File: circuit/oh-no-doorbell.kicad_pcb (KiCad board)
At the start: 2 copper layers, 3.6 x 3.4 mm, 2 parts, among them J2 Conn_VDG, U1 ATtiny4-TS

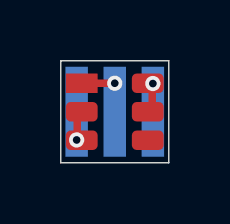
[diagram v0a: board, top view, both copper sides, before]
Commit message: Fix PCB
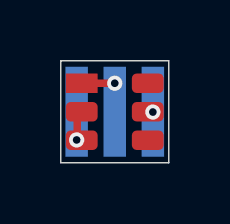
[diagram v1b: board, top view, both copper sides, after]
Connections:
- U1 pad 6: /BJT_C -> Net-(U1-Pad6)
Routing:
- net /BJT_C: track 1.07 -> 0.00 mm
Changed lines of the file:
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@@
     (thickness 0.2)
     (drawings 4)
-    (tracks 10)
+    (tracks 7)
     (zones 0)
     (modules 2)
-    (nets 5)
+    (nets 6)
   )
   (page A4)
@@
     (pad_to_mask_clearance 0)
     (aux_axis_origin 0 0)
-    (visible_elements 7FFFFFFF)
+    (visible_elements 7FFFFF7F)
     (pcbplotparams
       (layerselection 0x010fc_ffffffff)
@@
   (net 3 /BJT_E)
   (net 4 "Net-(U1-Pad4)")
+  (net 5 "Net-(U1-Pad6)")
   (net_class Default "This is the default net class."
     (clearance 0.2)
@@
     (add_net /BJT_E)
     (add_net "Net-(U1-Pad4)")
+    (add_net "Net-(U1-Pad6)")
   )
   (module Package_TO_SOT_SMD:SOT-23-6 (layer F.Cu)
@@
       (effects (font (size 1 1) (thickness 0.15)))
     )
-    (fp_line (start 0.9 -1.55) (end 0.9 1.55) (layer F.Fab) (width 0.1))
-    (fp_line (start 0.9 1.55) (end -0.9 1.55) (layer F.Fab) (width 0.1))
-    (fp_line (start -0.9 -0.9) (end -0.9 1.55) (layer F.Fab) (width 0.1))
-    (fp_line (start 0.9 -1.55) (end -0.25 -1.55) (layer F.Fab) (width 0.1))
-    (fp_line (start -0.9 -0.9) (end -0.25 -1.55) (layer F.Fab) (width 0.1))
-    (fp_line (start -1.9 -1.8) (end -1.9 1.8) (layer F.CrtYd) (width 0.05))
-    (fp_line (start -1.9 1.8) (end 1.9 1.8) (layer F.CrtYd) (width 0.05))
-    (fp_line (start 1.9 1.8) (end 1.9 -1.8) (layer F.CrtYd) (width 0.05))
-    (fp_line (start 1.9 -1.8) (end -1.9 -1.8) (layer F.CrtYd) (width 0.05))
     (fp_text user %R (at 0 0 90) (layer F.Fab) hide
       (effects (font (size 0.5 0.5) (thickness 0.075)))
     )
+    (fp_line (start 1.9 -1.8) (end -1.9 -1.8) (layer F.CrtYd) (width 0.05))
+    (fp_line (start 1.9 1.8) (end 1.9 -1.8) (layer F.CrtYd) (width 0.05))
+    (fp_line (start -1.9 1.8) (end 1.9 1.8) (layer F.CrtYd) (width 0.05))
+    (fp_line (start -1.9 -1.8) (end -1.9 1.8) (layer F.CrtYd) (width 0.05))
+    (fp_line (start -0.9 -0.9) (end -0.25 -1.55) (layer F.Fab) (width 0.1))
+    (fp_line (start 0.9 -1.55) (end -0.25 -1.55) (layer F.Fab) (width 0.1))
+    (fp_line (start -0.9 -0.9) (end -0.9 1.55) (layer F.Fab) (width 0.1))
+    (fp_line (start 0.9 1.55) (end -0.9 1.55) (layer F.Fab) (width 0.1))
+    (fp_line (start 0.9 -1.55) (end 0.9 1.55) (layer F.Fab) (width 0.1))
+    (pad 1 smd rect (at -1.1 -0.95) (size 1.06 0.65) (layers F.Cu F.Paste F.Mask)
+      (net 1 /BJT_B))
+    (pad 2 smd roundrect (at -1.1 0) (size 1.06 0.65) (layers F.Cu F.Paste F.Mask) (roundrect_rratio 0.25)
+      (net 3 /BJT_E))
+    (pad 3 smd roundrect (at -1.1 0.95) (size 1.06 0.65) (layers F.Cu F.Paste F.Mask) (roundrect_rratio 0.25)
+      (net 3 /BJT_E))
+    (pad 4 smd roundrect (at 1.1 0.95) (size 1.06 0.65) (layers F.Cu F.Paste F.Mask) (roundrect_rratio 0.25)
+      (net 4 "Net-(U1-Pad4)"))
+    (pad 6 smd roundrect (at 1.1 -0.95) (size 1.06 0.65) (layers F.Cu F.Paste F.Mask) (roundrect_rratio 0.25)
+      (net 5 "Net-(U1-Pad6)"))
     (pad 5 smd roundrect (at 1.1 0) (size 1.06 0.65) (layers F.Cu F.Paste F.Mask) (roundrect_rratio 0.25)
       (net 2 /BJT_C))
-    (pad 6 smd roundrect (at 1.1 -0.95) (size 1.06 0.65) (layers F.Cu F.Paste F.Mask) (roundrect_rratio 0.25)
-      (net 2 /BJT_C))
-    (pad 4 smd roundrect (at 1.1 0.95) (size 1.06 0.65) (layers F.Cu F.Paste F.Mask) (roundrect_rratio 0.25)
-      (net 4 "Net-(U1-Pad4)"))
-    (pad 3 smd roundrect (at -1.1 0.95) (size 1.06 0.65) (layers F.Cu F.Paste F.Mask) (roundrect_rratio 0.25)
-      (net 3 /BJT_E))
-    (pad 2 smd roundrect (at -1.1 0) (size 1.06 0.65) (layers F.Cu F.Paste F.Mask) (roundrect_rratio 0.25)
-      (net 3 /BJT_E))
-    (pad 1 smd rect (at -1.1 -0.95) (size 1.06 0.65) (layers F.Cu F.Paste F.Mask)
-      (net 1 /BJT_B))
     (model ${KISYS3DMOD}/Package_TO_SOT_SMD.3dshapes/SOT-23-6.wrl
       (at (xyz 0 0 0))
@@
     )
   )
+  (gr_line (start 101.8 98.3) (end 98.2 98.3) (layer Edge.Cuts) (width 0.05))
+  (gr_line (start 101.8 101.7) (end 101.8 98.3) (layer Edge.Cuts) (width 0.05))
+  (gr_line (start 98.2 101.7) (end 98.2 98.3) (layer Edge.Cuts) (width 0.05))
   (gr_line (start 101.8 101.7) (end 98.2 101.7) (layer Edge.Cuts) (width 0.05))
-  (gr_line (start 101.8 101.7) (end 101.8 98.3) (layer Edge.Cuts) (width 0.05))
-  (gr_line (start 101.8 98.3) (end 98.2 98.3) (layer Edge.Cuts) (width 0.05))
-  (gr_line (start 98.2 101.7) (end 98.2 98.3) (layer Edge.Cuts) (width 0.05))
-  (via (at 98.73003 100.94) (size 0.508) (drill 0.254) (layers F.Cu B.Cu) (net 3) (status 1000000))
-  (segment (start 98.75 100.15) (end 98.75 100.8) (width 0.25) (layer F.Cu) (net 3) (status 1000000))
-  (segment (start 98.9 100) (end 98.75 100.15) (width 0.25) (layer F.Cu) (net 3) (status 1000000))
-  (segment (start 98.75 100.8) (end 98.9 100.95) (width 0.25) (layer F.Cu) (net 3) (status 1000000))
   (via (at 100 99.05) (size 0.508) (drill 0.254) (layers F.Cu B.Cu) (net 1))
   (segment (start 98.9 99.05) (end 100 99.05) (width 0.25) (layer F.Cu) (net 1))
-  (segment (start 101.25 99.2) (end 101.1 99.05) (width 0.25) (layer F.Cu) (net 2) (status 1000000))
-  (segment (start 101.1 100) (end 101.25 99.85) (width 0.25) (layer F.Cu) (net 2) (status 1000000))
-  (via (at 101.26997 99.06) (size 0.508) (drill 0.254) (layers F.Cu B.Cu) (net 2) (status 1000000))
-  (segment (start 101.25 99.85) (end 101.25 99.2) (width 0.25) (layer F.Cu) (net 2) (status 1000000))
+  (via (at 101.26997 100.01) (size 0.508) (drill 0.254) (layers F.Cu B.Cu) (net 2))
+  (via (at 98.73003 100.94) (size 0.508) (drill 0.254) (layers F.Cu B.Cu) (net 3))
+  (segment (start 98.75 100.15) (end 98.75 100.8) (width 0.25) (layer F.Cu) (net 3))
+  (segment (start 98.9 100) (end 98.75 100.15) (width 0.25) (layer F.Cu) (net 3))
+  (segment (start 98.75 100.8) (end 98.9 100.95) (width 0.25) (layer F.Cu) (net 3))
 )
